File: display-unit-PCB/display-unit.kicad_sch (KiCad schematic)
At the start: 3 parts, among them J1 RJ45_LED_Shielded, J2 Display, J3 ESP32 38-Pin

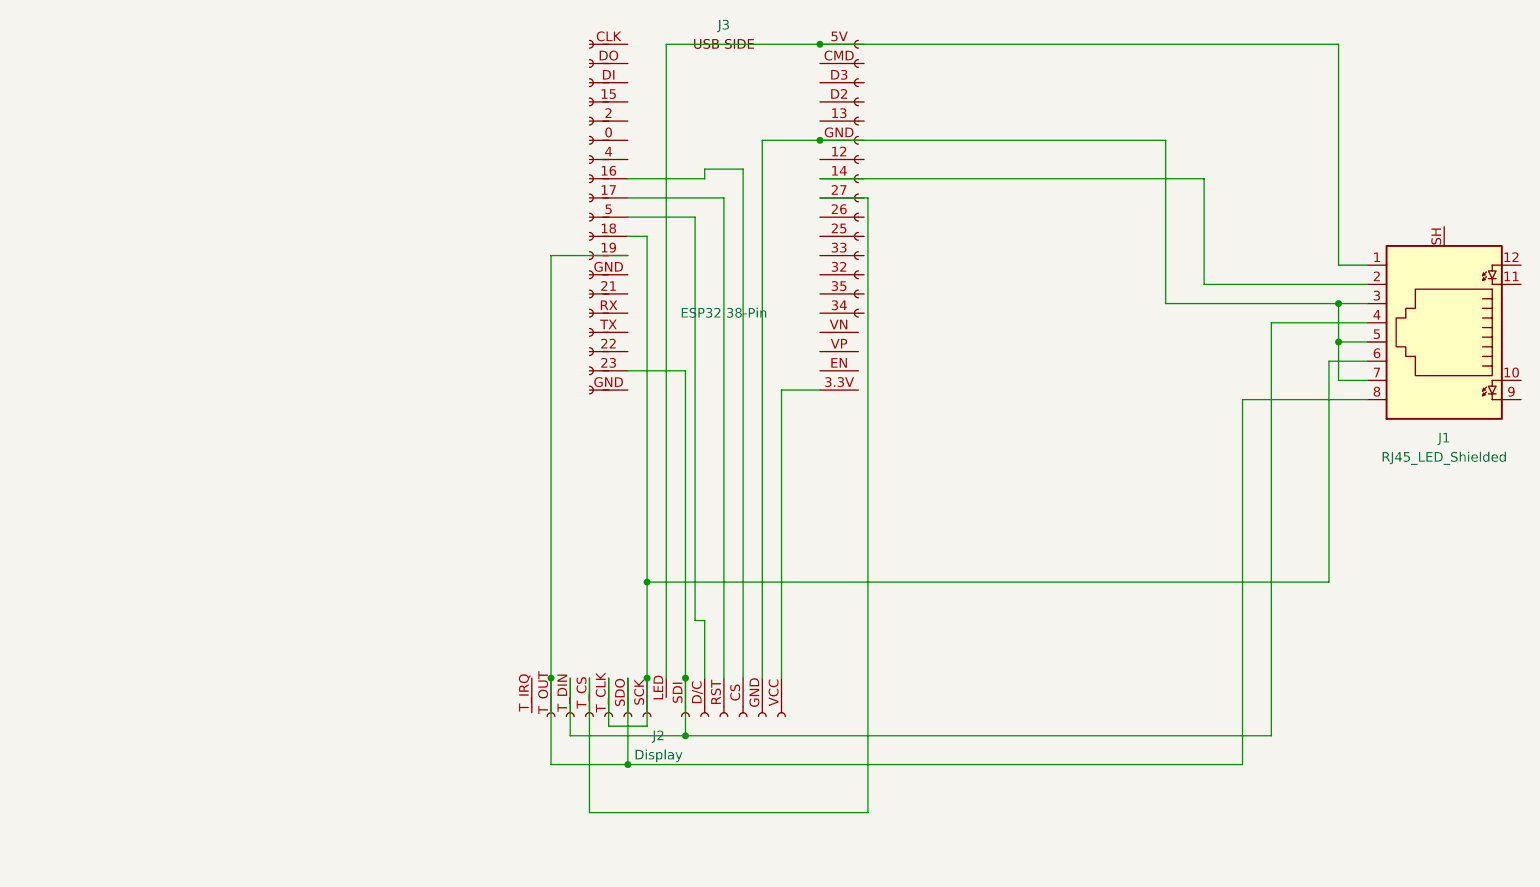
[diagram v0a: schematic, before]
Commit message: trying to migrate
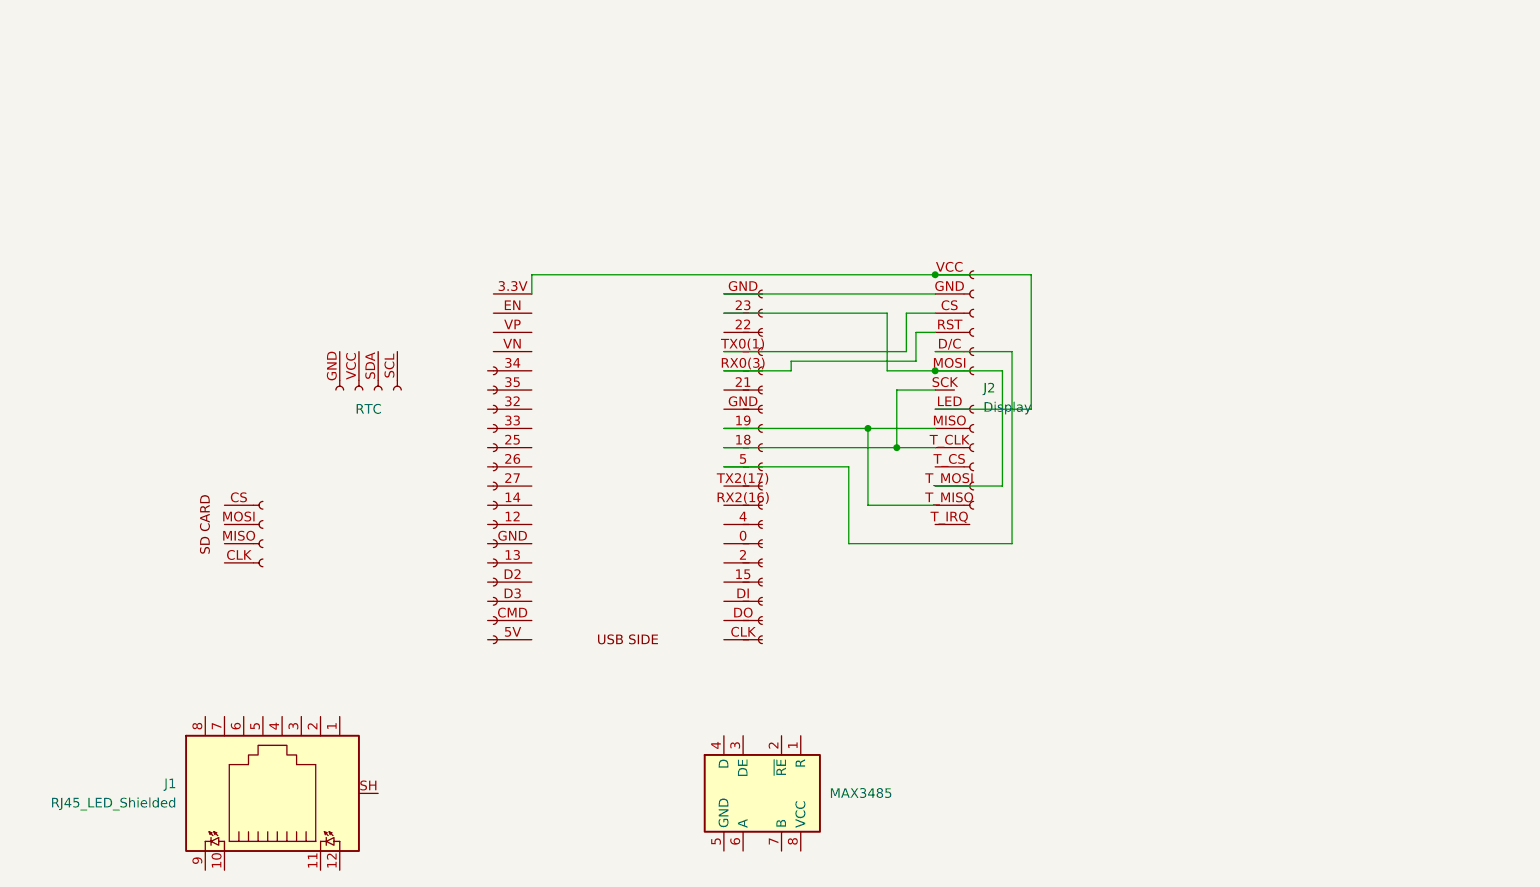
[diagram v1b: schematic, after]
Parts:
- added J4: SD_Card, Connector_PinSocket_2.54mm:PinSocket_1x04_P2.54mm_Vertical, symbol Connector:Conn_01x04_Socket
- added J5: RTC, Connector_PinSocket_2.54mm:PinSocket_1x04_P2.54mm_Vertical, symbol Connector:Conn_01x04_Socket
- added U1: MAX3485, Package_DIP:DIP-8_W7.62mm, symbol Interface_UART:SN75176AP
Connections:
- net at J1.2: no longer J3.14 (Pin_22)
- net at J2.SCK (14), J2.T_CLK (Pin_9), J3.18 (Pin_5): no longer J1.6
- net at J2.CS (Pin_3): now also J3.TX0(1) (Pin_2); no longer J3.16 (Pin_8)
- net at J2.RST (Pin_4): now also J3.RX0(3) (3.3); no longer J3.17 (Pin_7)
- net at J2.T_CS (Pin_10): no longer J3.27 (Pin_23)
- net at J2.VCC, J3.3.3V: now also J2.LED (Pin_7)
- new net: J2.GND (Pin_2), J3.GND (Pin_20)
- new net: J2.MISO (Pin_8), J2.T_MISO (Pin_12), J3.19 (Pin_4)
- new net: J2.MOSI (Pin_6), J2.T_MOSI (Pin_11), J3.23 (Pin_2)
- now unconnected: J1.1, J1.3, J1.4, J1.5, J1.7, J1.8, J3.5V (Pin_15), J3.GND (Pin_20)
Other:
- moved on the sheet: J1, J2
